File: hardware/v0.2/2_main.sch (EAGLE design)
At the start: 72 parts, among them IC1 SN74LVC1G08, IC2 FP6291, IC4 STM32F10XCXT6, J1 RJ9PTH, Q2 8050, Q3 MOSFET-NCHANNELBSS138, Q4 MOSFET-NCHANNELBSS138, Y1 8M

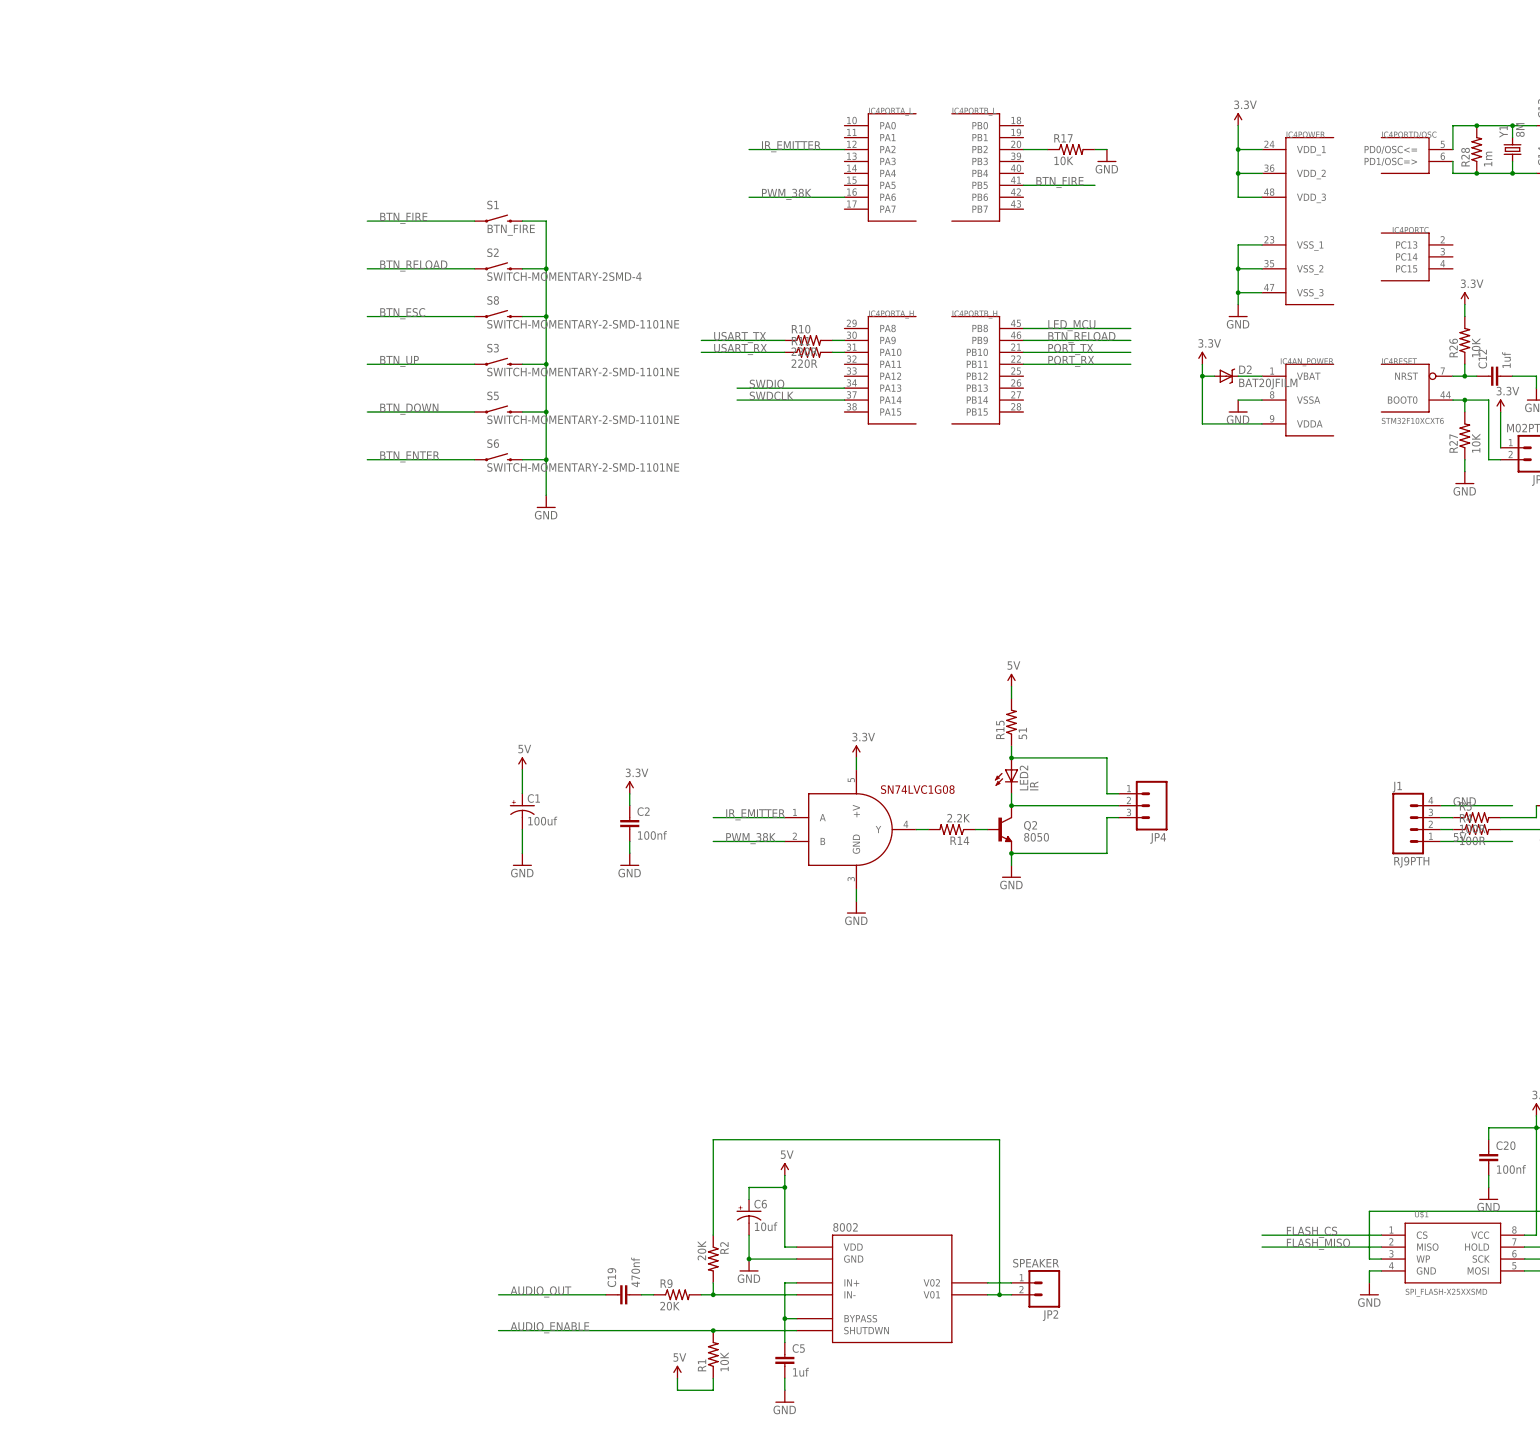
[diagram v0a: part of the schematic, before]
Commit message: update sch
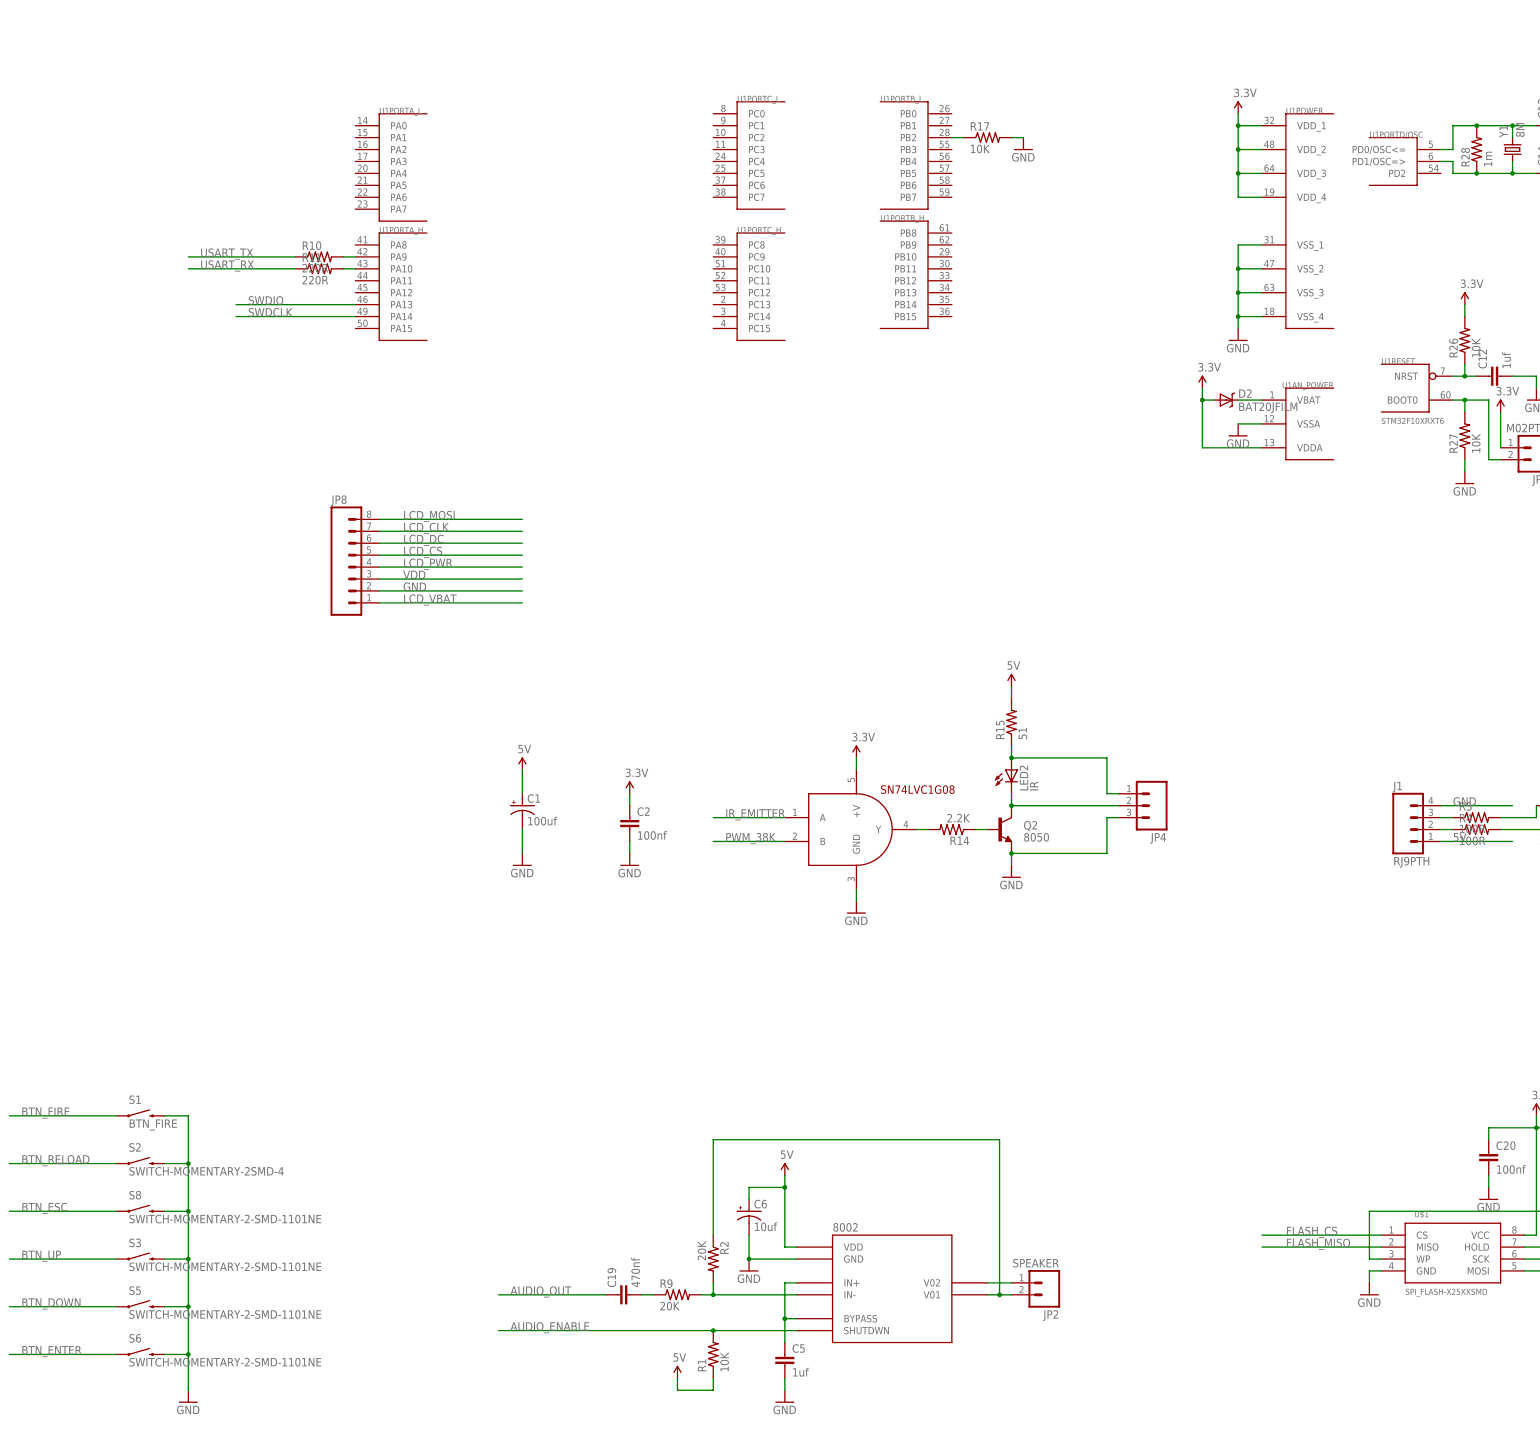
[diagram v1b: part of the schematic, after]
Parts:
- removed IC4: STM32F10XCXT6, stm32:STM32F10XCXT6
- added JP8: (no value), SparkFun-Connectors:M081X08
- added U1: STM32F10XRXT6, stm32:STM32F10XRXT6
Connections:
- removed net LED_MCU: IC4PORTB_H.PB8
- removed net N$37: IC4PORTA_H.PA9, R10.2
- removed net N$38: IC4PORTA_H.PA10, R11.2
- new net LCD_CLK: JP8.7
- new net LCD_CS: JP8.5
- new net LCD_DC: JP8.6
- new net LCD_MOSI: JP8.8
- new net LCD_PWR: JP8.4
- new net LCD_VBAT: JP8.1
- new net N$27: R10.2, U1PORTA_H.PA9
- new net N$28: R11.2, U1PORTA_H.PA10
- new net VDD: JP8.3
- net 3.3V: now also U1AN_POWER.VDDA, U1POWER.VDD_1, U1POWER.VDD_2, U1POWER.VDD_3, U1POWER.VDD_4; no longer IC4AN_POWER.VDDA, IC4POWER.VDD_1, IC4POWER.VDD_2, IC4POWER.VDD_3
- net BTN_FIRE: no longer IC4PORTB_L.PB5
- net BTN_RELOAD: no longer IC4PORTB_H.PB9
- net GND: now also JP8.2, U1AN_POWER.VSSA, U1POWER.VSS_1, U1POWER.VSS_2, U1POWER.VSS_3, U1POWER.VSS_4; no longer IC4AN_POWER.VSSA, IC4POWER.VSS_1, IC4POWER.VSS_2, IC4POWER.VSS_3
- net IR_EMITTER: no longer IC4PORTA_L.PA2
- net N$1: now also U1PORTB_L.PB2; no longer IC4PORTB_L.PB2
- net N$2: now also U1RESET.BOOT0; no longer IC4RESET.BOOT0
- net N$3: now also U1PORTD/OSC.PD0/OSC<=; no longer IC4PORTD/OSC.PD0/OSC<=
- net N$4: now also U1PORTD/OSC.PD1/OSC=>; no longer IC4PORTD/OSC.PD1/OSC=>
- net N$44: now also U1RESET.NRST; no longer IC4RESET.NRST
- net N$5: now also U1AN_POWER.VBAT; no longer IC4AN_POWER.VBAT
- net PORT_RX: no longer IC4PORTB_H.PB11
- net PORT_TX: no longer IC4PORTB_H.PB10
- net PWM_38K: no longer IC4PORTA_L.PA6
- net SWDCLK: now also U1PORTA_H.PA14; no longer IC4PORTA_H.PA14
- net SWDIO: now also U1PORTA_H.PA13; no longer IC4PORTA_H.PA13
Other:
- moved on the sheet: D2, R10, R11, R17, S1, S2, S3, S5, S6, S8

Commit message: update sch
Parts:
- removed JP3: M02PTH, SparkFun-Connectors:M02PTH
- removed JP4: (no value), SparkFun-Connectors:M03PTH
- added C22: 100nf, SparkFun-Passives:CAP0603-CAP
- added JP1: M02POLAR, SparkFun-Connectors:M02POLAR
- added Q5: 8550, SparkFun-DiscreteSemi:TRANSISTOR_PNPMMBT4403
- added R16: 51, SparkFun-Passives:RESISTOR0603-RES
- added R18: 1K, SparkFun-Passives:RESISTOR0603-RES
- added R21, R22: 0R, SparkFun-Passives:RESISTOR0603-RES
- added R23: 10K, SparkFun-Passives:RESISTOR0603-RES
- R15: value 51 -> 1K; device SparkFun-Resistors:RESISTOR1206 -> SparkFun-Passives:RESISTOR0603-RES
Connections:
- removed net FLASH_SCK: U$1.SCK
- removed net LCD_CS: JP8.5
- removed net LCD_VBAT: JP8.1
- new net FLASH_CLK: U$1.SCK, U1PORTB_H.PB13
- new net IR_EMMITER: U1PORTB_H.PB10
- new net N$29: Q5.B, R15.2, R23.1
- new net N$30: C22.1, R18.2, R21.1
- new net N$31: R22.2, U1PORTA_L.PA4
- new net N$32: JP8.1, Q5.C
- new net V_BATT: C3.1, C4.1, F1.2, IC2.EN, IC2.VCC, L1.1, Q5.E, R23.2
- net 5V: now also R16.2; no longer R15.2
- net AUDIO_OUT: now also R21.2, R22.1
- net FLASH_CS: now also U1PORTB_H.PB12
- net FLASH_MISO: now also U1PORTB_H.PB14
- net FLASH_MOSI: now also U1PORTB_H.PB15
- net GND: now also C22.2, JP1.1; no longer JP3.1, JP4.3
- net LCD_CLK: now also U1PORTA_L.PA5
- net LCD_DC: now also U1PORTA_L.PA6
- net LCD_MOSI: now also U1PORTA_L.PA7
- net LCD_PWR: now also R15.1, U1PORTB_H.PB11; no longer JP8.4
- net N$14: now also R18.1; no longer JP4.1, LED2.A, R15.1
- net N$20: now also LED2.A, R16.1; no longer C3.1, C4.1, F1.2, IC2.EN, IC2.VCC, L1.1
- net N$7: now also JP1.2; no longer JP3.2
- net N$8: no longer JP4.2
- net PORT_RX: now also U1PORTC_H.PC11
- net PORT_TX: now also U1PORTC_H.PC10
- net PWM_38K: now also U1PORTB_L.PB1
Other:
- moved on the sheet: C1, C2, J1, JP8, LED2, Q2, Q3, Q4, R14, R15, R3, R4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

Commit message: add mirco sd socket
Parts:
- removed JP8: (no value), SparkFun-Connectors:M081X08
- removed Q5: 8550, SparkFun-DiscreteSemi:TRANSISTOR_PNPMMBT4403
- removed R15: 1K, SparkFun-Passives:RESISTOR0603-RES
- added D3: 1N5819, SparkFun-DiscreteSemi:BAT20JFILM
- added JP3: (no value), SparkFun-Connectors:M06POLAR
- added Q1: PMOS, SparkFun-DiscreteSemi:MOSFET-PCHANNELSMD
- added SD1: MICROSD_YOUXIN, eagle_lib_lishen:MICROSD_YOUXIN
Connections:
- new net SD_CLK: SD1.CLK, U1PORTB_L.PB3
- new net SD_CS: SD1./CS, U1PORTB_L.PB6
- new net SD_MISO: SD1.DO, U1PORTB_L.PB4
- new net SD_MOSI: SD1.DI, U1PORTB_L.PB5
- net 3.3V: now also SD1.VDD
- net GND: now also JP3.2, SD1.VSS; no longer JP8.2
- net LCD_CLK: now also JP3.5; no longer JP8.7
- net LCD_DC: now also JP3.4; no longer JP8.6
- net LCD_MOSI: now also JP3.6; no longer JP8.8
- net LCD_PWR: now also Q1.G, R23.1; no longer R15.1
- net N$29: now also D3.C, JP3.1; no longer Q5.B, R15.2, R23.1
- net N$32: now also D3.A, Q1.D; no longer JP8.1, Q5.C
- net VDD: now also JP3.3; no longer JP8.3
- net V_BATT: now also Q1.S; no longer Q5.E
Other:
- moved on the sheet: C22, R21, R23
